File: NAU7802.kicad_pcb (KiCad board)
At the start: 2 copper layers, 22.1 x 33.5 mm, 17 parts, among them J1 A Scale, J2 B scale, J3 I²C, J4 Scale, U1 NAU7802SGI

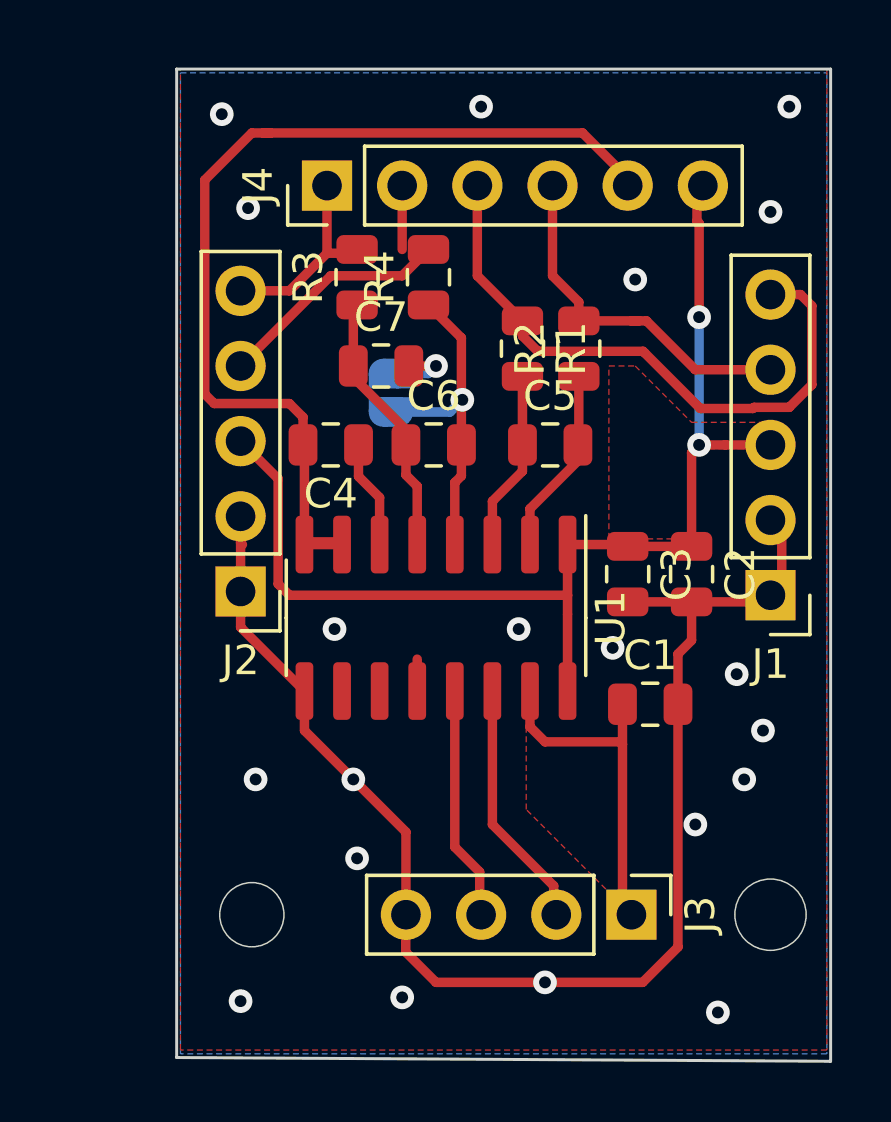
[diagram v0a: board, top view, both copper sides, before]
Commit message: Add files via upload
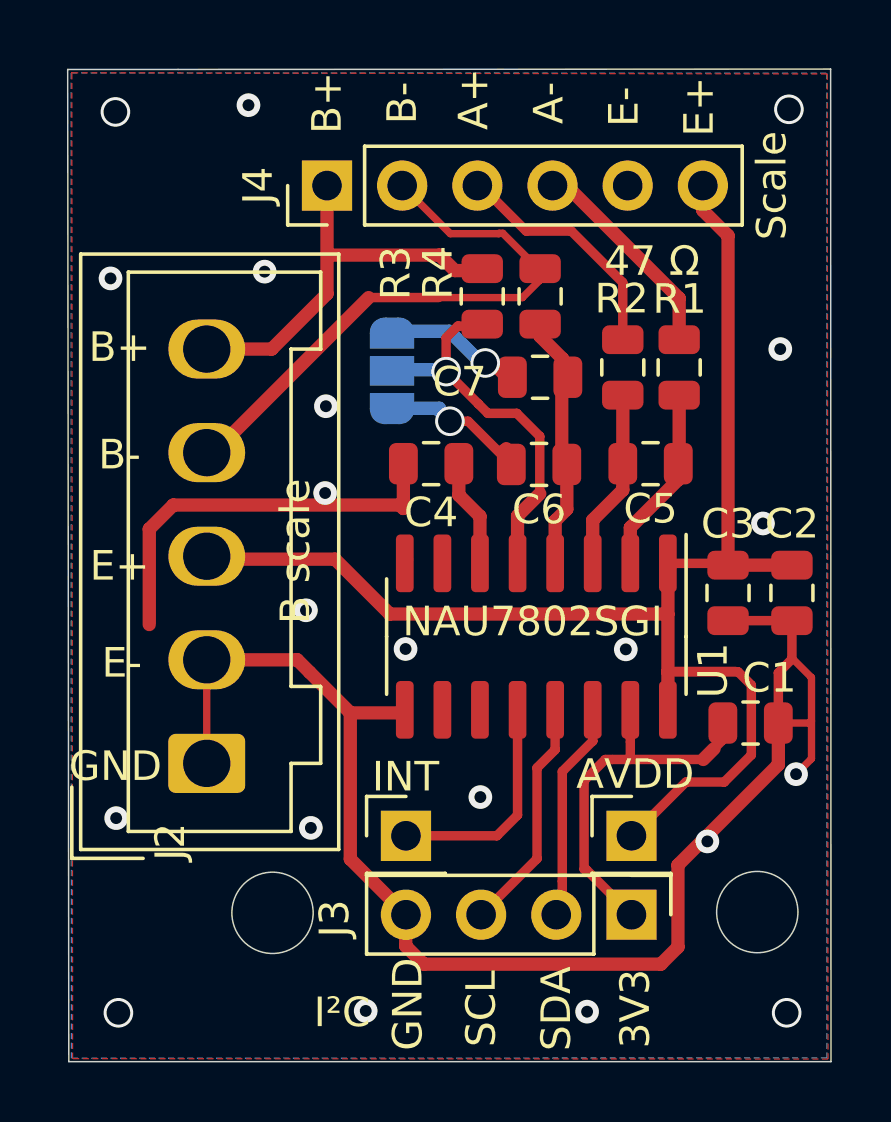
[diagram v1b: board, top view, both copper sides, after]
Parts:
- removed J1: A Scale, Connector_PinHeader_2.54mm:PinHeader_1x05_P2.54mm_Vertical
- added G***: LOGO, KiCad:Hiveeyes_Logo, B.Cu at (52.6, 49.7)
- added J5: AVDD, Connector_PinHeader_2.54mm:PinHeader_1x01_P2.54mm_Vertical, F.Cu at (49.8, 53.8)
- added J6: INT, Connector_PinHeader_2.54mm:PinHeader_1x01_P2.54mm_Vertical, F.Cu at (42.2, 53.8)
- added REF**: OSHW-Logo2_7.3x6mm_SilkScreen, KiCad:OSHW-Logo2_7.3x6mm_SilkScreen, B.Cu at (34.3, 58.4)
- J2: footprint Connector_PinHeader_2.54mm:PinHeader_1x05_P2.54mm_Vertical -> Connector_Wago:Wago_734-135_1x05_P3.50mm_Vertical
- JP1: value B Disabe -> en; footprint Jumper:SolderJumper-2_P1.3mm_Open_RoundedPad1.0x1.5mm -> Jumper:SolderJumper-3_P1.3mm_Open_RoundedPad1.0x1.5mm
- R1: value R1-4=47 Ω -> 47 Ω
- moved J2 5.92 mm to (35.4, 51.4), turned to 90 degrees
- moved C7 5.39 mm to (46.7, 38.4)
- moved R3 4.28 mm to (44.7, 35.6)
- moved R4 3.83 mm to (46.7, 35.6)
- moved C6 3.62 mm to (46.7, 41.3)
- moved R1 3.45 mm to (49.5, 38.0)
- moved R2 3.45 mm to (51.4, 38.0)
- moved C1 3.45 mm to (53.8, 50.0)
- moved C3 3.45 mm to (53.0, 45.6)
- moved C5 3.45 mm to (50.4, 41.3)
- moved U1 3.45 mm to (46.6, 47.1)
- moved C2 3.45 mm to (55.2, 45.6)
- moved C4 3.45 mm to (43.0, 41.3)
- moved JP1 0.74 mm to (41.7, 38.1)
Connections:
- C7 pad 1: Net-(C6-Pad1) -> Net-(C7-Pad1)
- C7 pad 2: Net-(C7-Pad2) -> Net-(C6-Pad2)
- JP1 pad 1: Net-(C7-Pad2) -> Net-(C7-Pad1)
- JP1 pad 2: Net-(C6-Pad2) -> Net-(JP1-Pad2)
- R3 pad 1: Net-(C6-Pad1) -> Net-(JP1-Pad2)
- U1 pad 5: Net-(C6-Pad1) -> Net-(JP1-Pad2)
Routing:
- net AVDD: track 39.8 -> 57.3 mm, vias 2 -> 0
- net A+: track 21.1 -> 8.20 mm
- net Net-(JP1-Pad2): track 0.00 -> 12.4 mm, vias 0 -> 1
- net AVSS: track 80.8 -> 68.5 mm, vias 20 -> 21
- net B-: track 10.3 -> 22.4 mm
- net B+: track 6.80 -> 16.7 mm
- net INT: track 1.08 -> 7.62 mm
- net SCL: track 8.03 -> 14.6 mm
- net A-: track 12.9 -> 7.42 mm
- net Net-(C7-Pad1): track 0.00 -> 3.87 mm, vias 0 -> 1
- net Net-(C6-Pad1): track 10.3 -> 6.77 mm, vias 0 -> 1
- net DVDD: track 12.1 -> 15.4 mm
- net Net-(C6-Pad2): track 12.0 -> 9.26 mm, vias 1 -> 0
- net Net-(C7-Pad2): track 2.55 -> 0.00 mm, vias 1 -> 0
- removed copper zone on F.Cu, net AVDD
- removed copper zone on F.Cu, net DVDD
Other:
- board size 22.1 x 33.5 mm -> 25.8 x 33.5 mm
- board text added: "AVDD"
- board text added: "Hiveeyes.org NAU7802 V.1.0.0"
- board text added: "INT"
- board text added: "d"
